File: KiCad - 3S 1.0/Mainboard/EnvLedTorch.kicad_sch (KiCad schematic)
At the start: 133 parts, among them IC1 BQ25792RQMR, IC2 TPS25750DRJKR, J1 HRO_TYPE-C-31-M-12, J10 3S/1.5MHz/1A ICGH, J11 4S/1.5MHz/1A ICGH, J2 Conn_01x02, J3 Aardvark, J4 SYS/GND, J5 BAT/GND, J6 Aardvark, J7 THERMISTOR / GND, J8 TS/NORM, J9 2S/1.5MHz/2A ICGH, Q1 BSP89, Q2 BSP89, Q3 BSP89, Q4 AO3401A, Q5 AO3401A, U1 HY2213, U2 HY2213, U3 HY2213, U4 TLV75533PDBV, U5 TVS2200DRV, U6 CAT24C256, U9 8254

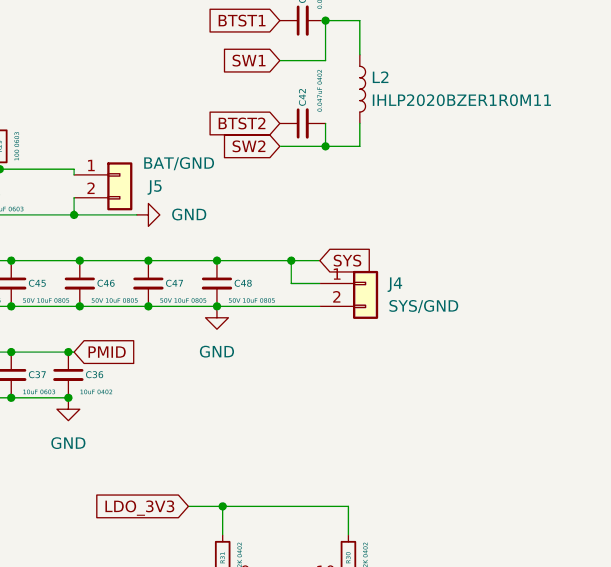
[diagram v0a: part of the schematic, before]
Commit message: few small corrections i forgot to commit
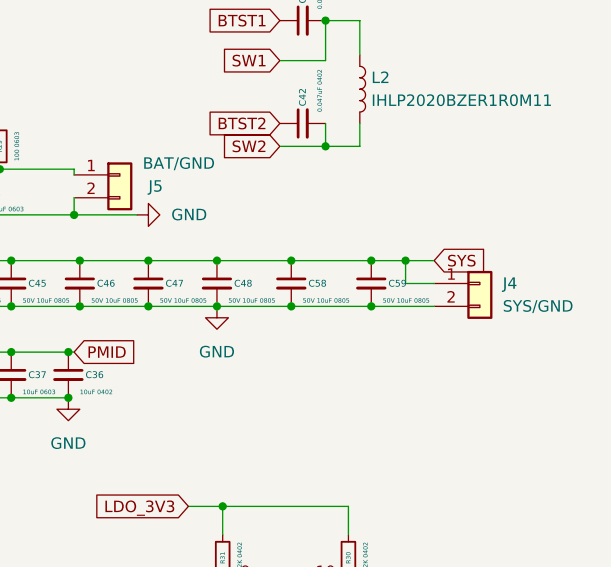
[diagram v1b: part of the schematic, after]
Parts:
- added C58, C59: 50V 10uF 0805, Capacitor_SMD:C_0805_2012Metric, symbol Device:C_Small
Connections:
- net GND: now also C58.2, C59.2
- net SYS: now also C58.1, C59.1
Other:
- moved on the sheet: J4
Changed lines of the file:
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@@
   (junction (at 368.935 157.48) (diameter 0) (color 0 0 0 0)
   )
+  (junction (at 385.445 127) (diameter 0) (color 0 0 0 0)
+  )
   (junction (at 147.955 97.155) (diameter 0) (color 0 0 0 0)
   )
@@
   (junction (at 147.955 92.075) (diameter 0) (color 0 0 0 0)
   )
+  (junction (at 385.445 121.92) (diameter 0) (color 0 0 0 0)
+  )
   (junction (at 102.235 263.525) (diameter 0) (color 0 0 0 0)
   )
@@
   (junction (at 381 28.575) (diameter 0) (color 0 0 0 0)
   )
-  (junction (at 376.555 121.92) (diameter 0) (color 0 0 0 0)
+  (junction (at 389.255 121.92) (diameter 0) (color 0 0 0 0)
   )
   (junction (at 389.89 28.575) (diameter 0) (color 0 0 0 0)
@@
   (junction (at 67.945 24.765) (diameter 0) (color 0 0 0 0)
   )
+  (junction (at 376.555 127) (diameter 0) (color 0 0 0 0)
+  )
   (junction (at 162.56 127.635) (diameter 0) (color 0 0 0 0)
   )
@@
   (junction (at 311.785 171.45) (diameter 0) (color 0 0 0 0)
   )
+  (junction (at 376.555 121.92) (diameter 0) (color 0 0 0 0)
+  )
   (junction (at 81.28 248.285) (diameter 0) (color 0 0 0 0)
   )
@@
     (stroke (width 0) (type default))
   )
-  (wire (pts (xy 376.555 121.92) (xy 368.3 121.92))
-    (stroke (width 0) (type default))
-  )
   (wire (pts (xy 372.11 197.485) (xy 372.11 194.31))
     (stroke (width 0) (type default))
@@
     (stroke (width 0) (type default))
   )
-  (wire (pts (xy 379.73 121.92) (xy 376.555 121.92))
+  (wire (pts (xy 392.43 121.92) (xy 389.255 121.92))
     (stroke (width 0) (type default))
   )
@@
     (stroke (width 0) (type default))
   )
-  (wire (pts (xy 379.73 124.46) (xy 376.555 124.46))
+  (wire (pts (xy 392.43 124.46) (xy 389.255 124.46))
     (stroke (width 0) (type default))
   )
@@
     (stroke (width 0) (type default))
   )
+  (wire (pts (xy 385.445 121.92) (xy 389.255 121.92))
+    (stroke (width 0) (type default))
+  )
   (wire (pts (xy 214.63 76.835) (xy 198.12 76.835))
     (stroke (width 0) (type default))
@@
     (stroke (width 0) (type default))
   )
-  (wire (pts (xy 376.555 124.46) (xy 376.555 121.92))
+  (wire (pts (xy 389.255 124.46) (xy 389.255 121.92))
     (stroke (width 0) (type default))
   )
@@
     (stroke (width 0) (type default))
   )
+  (wire (pts (xy 368.3 121.92) (xy 376.555 121.92))
+    (stroke (width 0) (type default))
+  )
   (wire (pts (xy 266.065 167.005) (xy 266.7 167.005))
     (stroke (width 0) (type default))
@@
     (stroke (width 0) (type default))
   )
+  (wire (pts (xy 376.555 127) (xy 385.445 127))
+    (stroke (width 0) (type default))
+  )
   (wire (pts (xy 271.78 129.54) (xy 282.575 129.54))
     (stroke (width 0) (type default))
@@
     (stroke (width 0) (type default))
   )
+  (wire (pts (xy 385.445 127) (xy 392.43 127))
+    (stroke (width 0) (type default))
+  )
   (wire (pts (xy 334.645 38.735) (xy 361.95 38.735))
     (stroke (width 0) (type default))
@@
     (stroke (width 0) (type default))
   )
+  (wire (pts (xy 368.3 127) (xy 376.555 127))
+    (stroke (width 0) (type default))
+  )
   (wire (pts (xy 270.51 177.8) (xy 266.7 177.8))
     (stroke (width 0) (type default))
@@
     (stroke (width 0) (type default))
   )
-  (wire (pts (xy 368.3 127) (xy 379.73 127))
-    (stroke (width 0) (type default))
-  )
   (wire (pts (xy 180.34 226.695) (xy 166.37 226.695))
     (stroke (width 0) (type default))
@@
     (stroke (width 0) (type default))
   )
+  (wire (pts (xy 376.555 121.92) (xy 385.445 121.92))
+    (stroke (width 0) (type default))
+  )
   (wire (pts (xy 43.18 42.545) (xy 45.72 42.545))
     (stroke (width 0) (type default))
@@
     )
   )
-  (global_label "SYS" (shape input) (at 379.73 121.92 0) (fields_autoplaced)
+  (global_label "SYS" (shape input) (at 392.43 121.92 0) (fields_autoplaced)
     (effects (font (size 1.27 1.27)) (justify left))
-    (property "Intersheetrefs" "${INTERSHEET_REFS}" (at 386.2228 121.92 0)
+    (property "Intersheetrefs" "${INTERSHEET_REFS}" (at 398.9228 121.92 0)
       (effects (font (size 1.27 1.27)) (justify left) hide)
     )
@@
     )
   )
+  (symbol (lib_id "Device:C_Small") (at 385.445 124.46 0) (unit 1)
+    (in_bom yes) (on_board yes) (dnp no)
+    (property "Reference" "C59" (at 387.35 124.46 0)
+      (effects (font (size 0.75 0.75)) (justify left))
+    )
+    (property "Value" "50V 10uF 0805" (at 386.715 126.365 0)
+      (effects (font (size 0.5 0.5)) (justify left))
+    )
+    (property "Footprint" "Capacitor_SMD:C_0805_2012Metric" (at 385.445 124.46 0)
+      (effects (font (size 1.27 1.27)) hide)
+    )
+    (property "Datasheet" "~" (at 385.445 124.46 0)
+      (effects (font (size 1.27 1.27)) hide)
+    )
+    (pin "1")
+    (pin "2")
+    (instances
+      (project "EnvLedTorch"
+        (path "/d80cef19-75ee-4cfe-8d31-e56b6cad8d97"
+          (reference "C59") (unit 1)
+        )
+      )
+    )
+  )
   (symbol (lib_id "power:GND") (at 272.415 119.38 0) (unit 1)
     (in_bom yes) (on_board yes) (dnp no) (fields_autoplaced)
@@
     )
   )
+  (symbol (lib_id "Device:C_Small") (at 376.555 124.46 0) (unit 1)
+    (in_bom yes) (on_board yes) (dnp no)
+    (property "Reference" "C58" (at 378.46 124.46 0)
+      (effects (font (size 0.75 0.75)) (justify left))
+    )
+    (property "Value" "50V 10uF 0805" (at 377.825 126.365 0)
+      (effects (font (size 0.5 0.5)) (justify left))
+    )
+    (property "Footprint" "Capacitor_SMD:C_0805_2012Metric" (at 376.555 124.46 0)
+      (effects (font (size 1.27 1.27)) hide)
+    )
+    (property "Datasheet" "~" (at 376.555 124.46 0)
+      (effects (font (size 1.27 1.27)) hide)
+    )
+    (pin "1")
+    (pin "2")
+    (instances
+      (project "EnvLedTorch"
+        (path "/d80cef19-75ee-4cfe-8d31-e56b6cad8d97"
+          (reference "C58") (unit 1)
+        )
+      )
+    )
+  )
   (symbol (lib_id "Transistor_FET:AO3401A") (at 58.42 196.85 270) (mirror x) (unit 1)
     (in_bom yes) (on_board yes) (dnp no) (fields_autoplaced)
@@
     )
   )
-  (symbol (lib_id "Connector_Generic:Conn_01x02") (at 384.81 124.46 0) (unit 1)
+  (symbol (lib_id "Connector_Generic:Conn_01x02") (at 397.51 124.46 0) (unit 1)
     (in_bom yes) (on_board yes) (dnp no) (fields_autoplaced)
-    (property "Reference" "J4" (at 387.35 124.46 0)
+    (property "Reference" "J4" (at 400.05 124.46 0)
       (effects (font (size 1.27 1.27)) (justify left))
     )
-    (property "Value" "SYS/GND" (at 387.35 127 0)
+    (property "Value" "SYS/GND" (at 400.05 127 0)
       (effects (font (size 1.27 1.27)) (justify left))
     )
-    (property "Footprint" "Connector_PinHeader_2.54mm:PinHeader_1x02_P2.54mm_Vertical" (at 384.81 124.46 0)
+    (property "Footprint" "Connector_PinHeader_2.54mm:PinHeader_1x02_P2.54mm_Vertical" (at 397.51 124.46 0)
       (effects (font (size 1.27 1.27)) hide)
     )
-    (property "Datasheet" "~" (at 384.81 124.46 0)
+    (property "Datasheet" "~" (at 397.51 124.46 0)
       (effects (font (size 1.27 1.27)) hide)
     )
